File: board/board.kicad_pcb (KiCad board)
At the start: 2 copper layers, 100 x 64 mm, 16 parts, among them J1 RJ12, J10 PLAN, J11 REMOTE_DISPLAY, J12 Conn_01x05_Socket, J13 RJ12, J14 JST PLAN, J15 REMOTE_DISPLAY, J16 RJ12, J2 JST XH, J3 JST XH, J4 RJ12, J5 Barrel_Jack, J6 Seriale, J7 MPX, J8 Conn_02x10_Counter_Clockwise_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, J9 Seriale

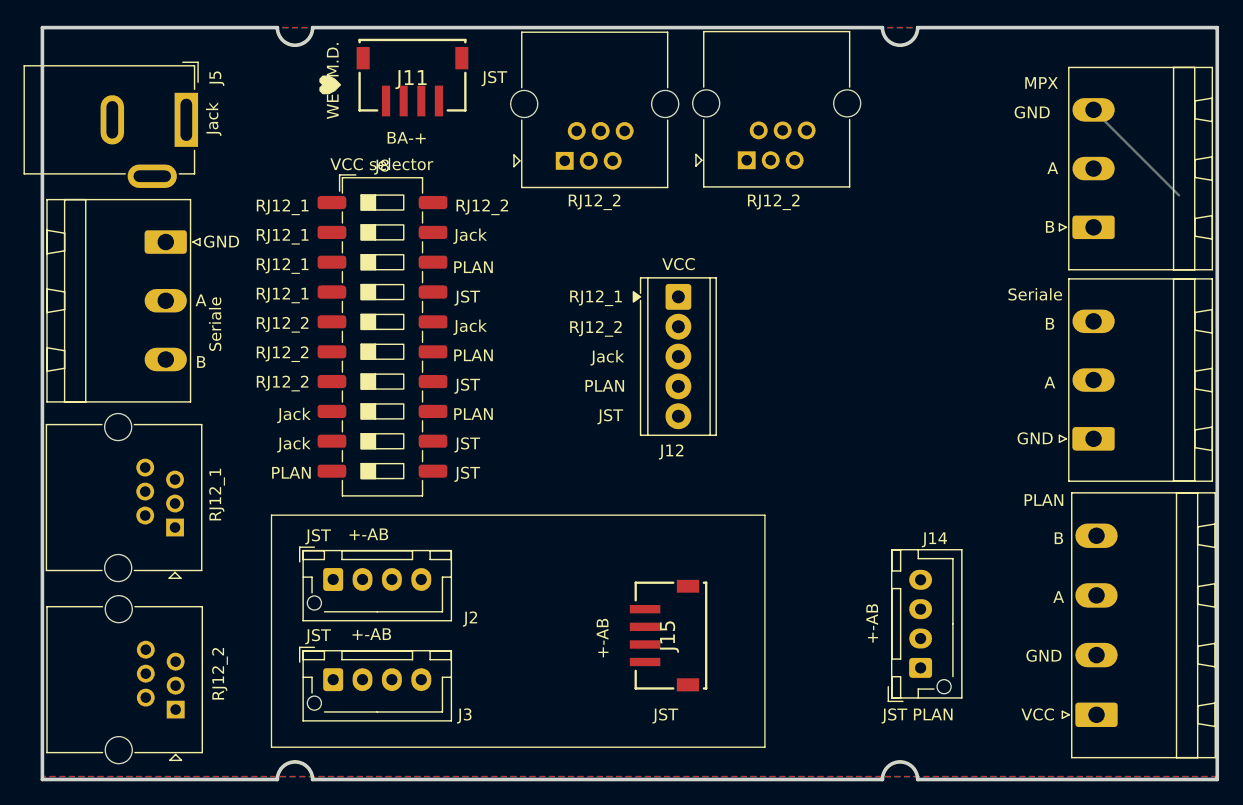
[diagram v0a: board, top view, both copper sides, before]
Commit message: [UPD] Update image
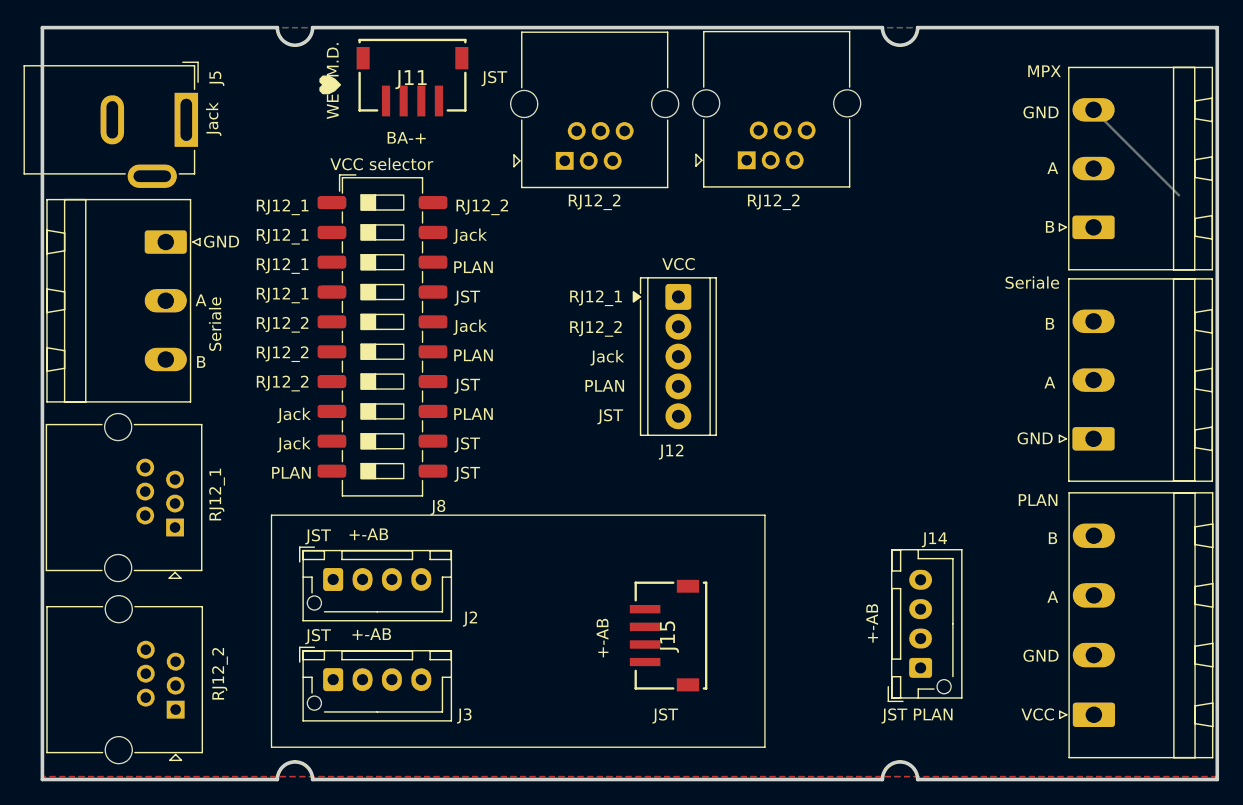
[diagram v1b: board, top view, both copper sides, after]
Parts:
- moved J10 0.22 mm to (181.0, 109.0)
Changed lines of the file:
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@@
 	(footprint "Connector_Phoenix_MSTB:PhoenixContact_MSTBA_2,5_4-G-5,08_1x04_P5.08mm_Horizontal"
 		(layer "F.Cu")
-		(at 181.2225 108.99 90)
+		(at 181 108.99 90)
 		(descr "Generic Phoenix Contact connector footprint for: MSTBA_2,5/4-G-5,08; number of pins: 04; pin pitch: 5.08mm; Angled || order number: 1757268 12A || order number: 1923885 16A (HC)")
 		(tags "phoenix_contact connector MSTBA_01x04_G_5.08mm")
@@
 		(tags "SMD DIP Switch SPST Slide 8.61mm 338mil SMD LowProfile")
 		(property "Reference" "J8"
-			(at 0 -14.54 0)
+			(at 4.805 14.43 0)
 			(layer "F.SilkS")
 			(effects
@@
 		)
 		(property "Value" "MPX"
-			(at 12.25 -4.4725 0)
+			(at 13.25 -4.2225 0)
 			(layer "F.SilkS")
 			(effects
@@
 		)
 		(property "Value" "Seriale"
-			(at 12.25 -4.9725 180)
+			(at 13.25 -5.2225 180)
 			(layer "F.SilkS")
 			(effects
@@
 	)
 	(gr_text "GND\n"
-		(at 175.75 57.75 0)
+		(at 176.5 57.75 0)
 		(layer "F.SilkS")
 		(effects
@@
 	)
 	(gr_text "PLAN\n"
-		(at 176.75 90.75 0)
+		(at 176.25 90.75 0)
 		(layer "F.SilkS")
 		(effects
@@
 	)
 	(gr_text "B"
-		(at 178 94 0)
+		(at 177.5 94 0)
 		(layer "F.SilkS")
 		(effects
@@
 	)
 	(gr_text "GND"
-		(at 176.75 104 0)
+		(at 176.5 104 0)
 		(layer "F.SilkS")
 		(effects
@@
 	)
 	(gr_text "A"
-		(at 178 99 0)
+		(at 177.5 99 0)
 		(layer "F.SilkS")
 		(effects
